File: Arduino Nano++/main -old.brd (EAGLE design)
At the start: 83.2 x 53.3 mm, 64 parts, among them IC1 LM358N, Q1 IRF9530, Q2 IRF9530

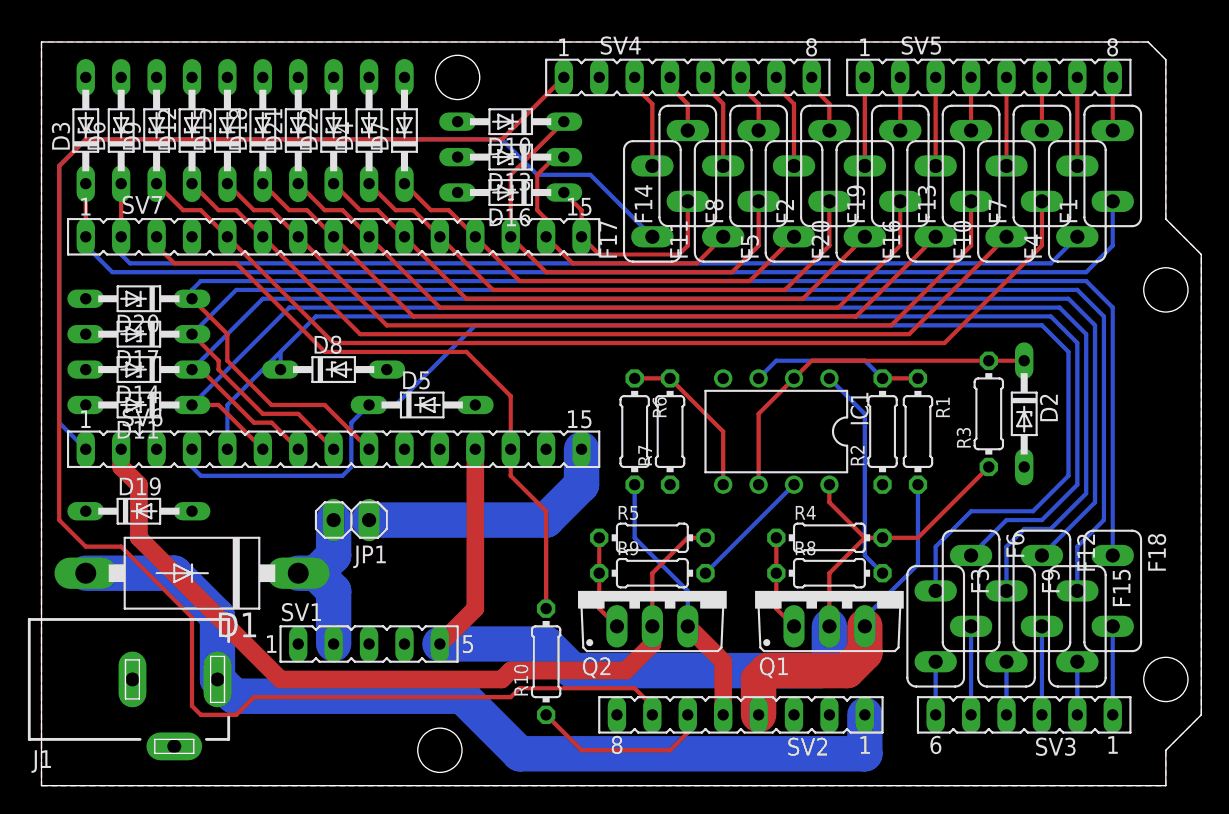
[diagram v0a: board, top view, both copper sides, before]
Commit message: Made version 2 of Nano++
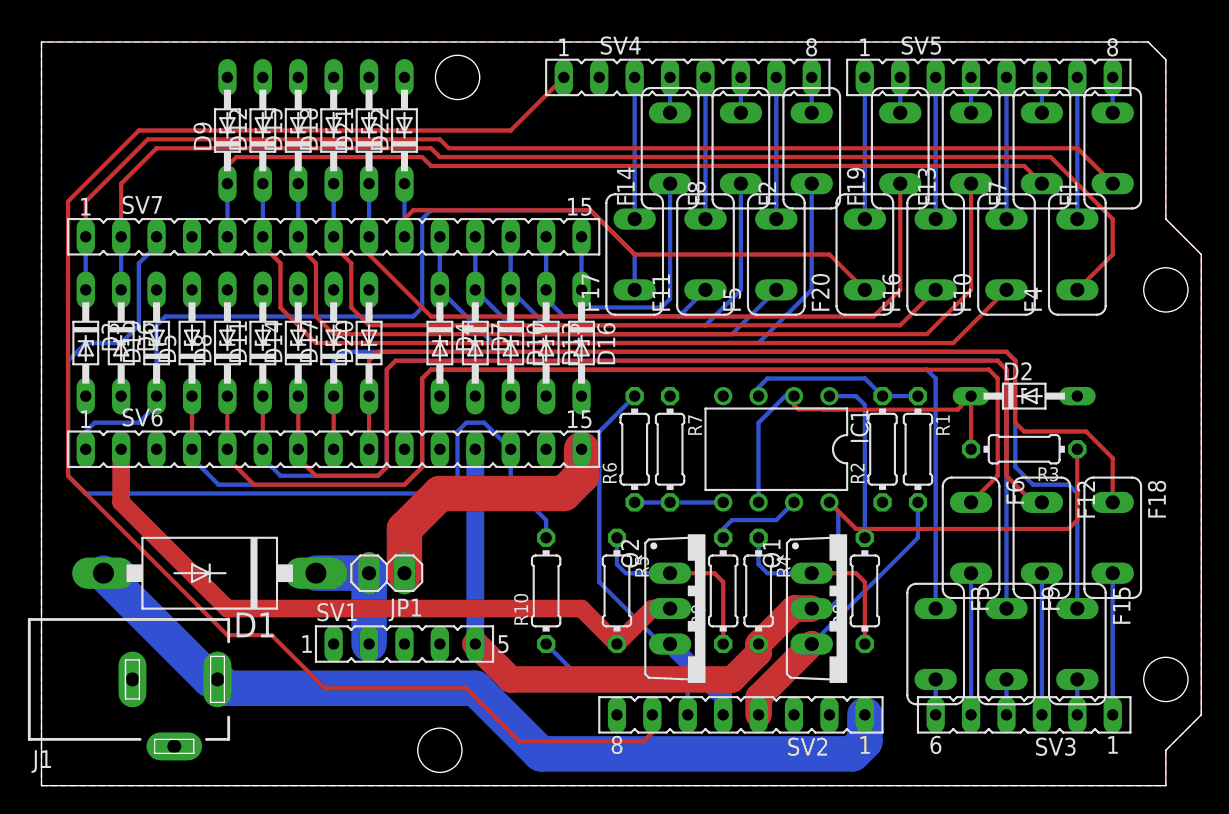
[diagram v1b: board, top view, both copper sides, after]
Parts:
- moved D5 17.1 mm to (11.4, 52.1), turned to 90 degrees
- moved D20 16.8 mm to (24.1, 52.1), turned to 90 degrees
- moved D4 16.1 mm to (29.2, 52.1), turned to 270 degrees
- moved D7 16.1 mm to (31.8, 52.1), turned to 270 degrees
- moved D10 15.9 mm to (34.3, 52.1), turned to 270 degrees
- moved D3 15.2 mm to (3.81, 52.1), turned to 270 degrees
- moved D6 15.2 mm to (6.35, 52.1), turned to 270 degrees
- moved D17 14.0 mm to (21.6, 52.1), turned to 90 degrees
- moved D13 13.6 mm to (36.8, 52.1), turned to 270 degrees
- moved D19 12.1 mm to (8.89, 52.1), turned to 90 degrees
- moved D16 11.9 mm to (39.4, 52.1), turned to 270 degrees
- moved D14 11.6 mm to (19.1, 52.1), turned to 90 degrees
- moved D11 9.94 mm to (16.5, 52.1), turned to 90 degrees
- moved D8 7.85 mm to (14.0, 52.1), turned to 90 degrees
- moved R4 6.35 mm to (52.1, 34.3), turned to 270 degrees
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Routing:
- net A5: track 103.8 -> 68.9 mm
- net A4: track 101.9 -> 76.9 mm
- net A3: track 95.7 -> 74.5 mm
- net RST: track 46.8 -> 65.7 mm
- net D1: track 74.7 -> 88.0 mm
- net A2: track 96.1 -> 83.2 mm
- net A0: track 95.2 -> 82.5 mm
- net A1: track 88.7 -> 77.6 mm
- net 3V3: track 58.9 -> 48.4 mm
- net D2: track 74.3 -> 64.6 mm
- net D13: track 67.3 -> 58.1 mm
- net 3V3': track 19.1 -> 28.0 mm
- net AREF': track 118.2 -> 110.3 mm
- net N$3: track 6.88 -> 14.5 mm
- net N$4: track 6.88 -> 14.5 mm
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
